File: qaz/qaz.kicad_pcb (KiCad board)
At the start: 2 copper layers, 227.4 x 57.3 mm, 49 parts, among them J1 OLED-128x32, SW1 SW_Push, SW10 SW_Push, SW11 SW_Push, SW12 SW_Push, SW13 SW_Push, SW14 SW_Push, SW15 SW_Push, SW16 SW_Push, SW17 SW_Push, SW18 SW_Push, SW19 SW_Push, SW2 SW_Push, SW20 SW_Push, SW21 SW_Push, SW22 SW_Push, SW23 SW_Push, SW24 SW_Push, SW25 SW_Push, SW26 SW_Push, SW27 SW_Push, SW28 SW_Push, SW3 SW_Push, SW4 SW_Push, SW5 SW_Push, SW6 SW_Push, SW7 SW_Push, SW8 SW_Push, SW9 SW_Push, U1 rp2040-zero

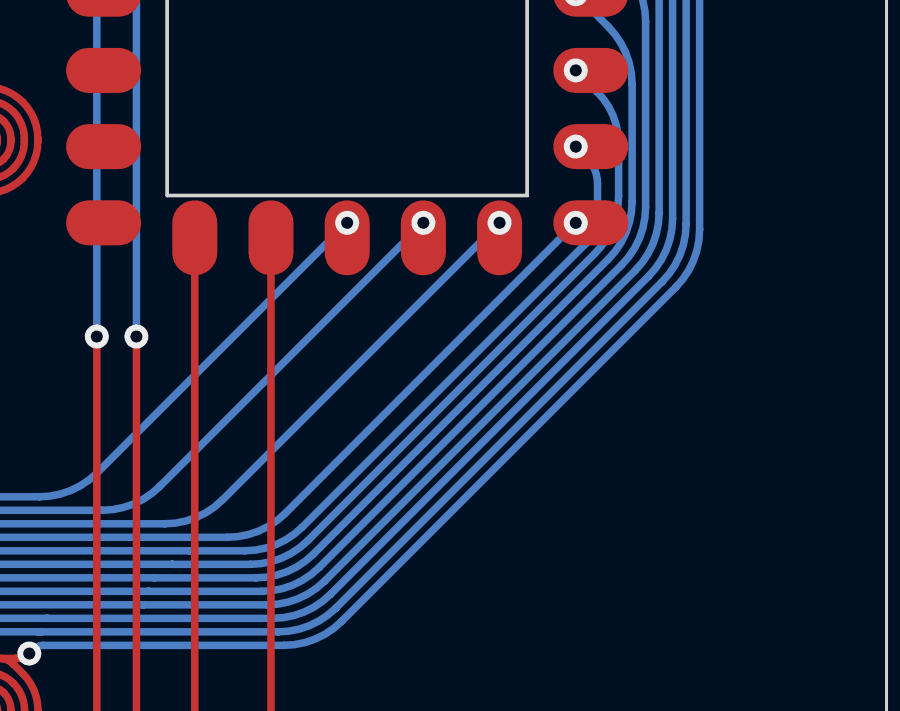
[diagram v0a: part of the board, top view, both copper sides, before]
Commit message: .
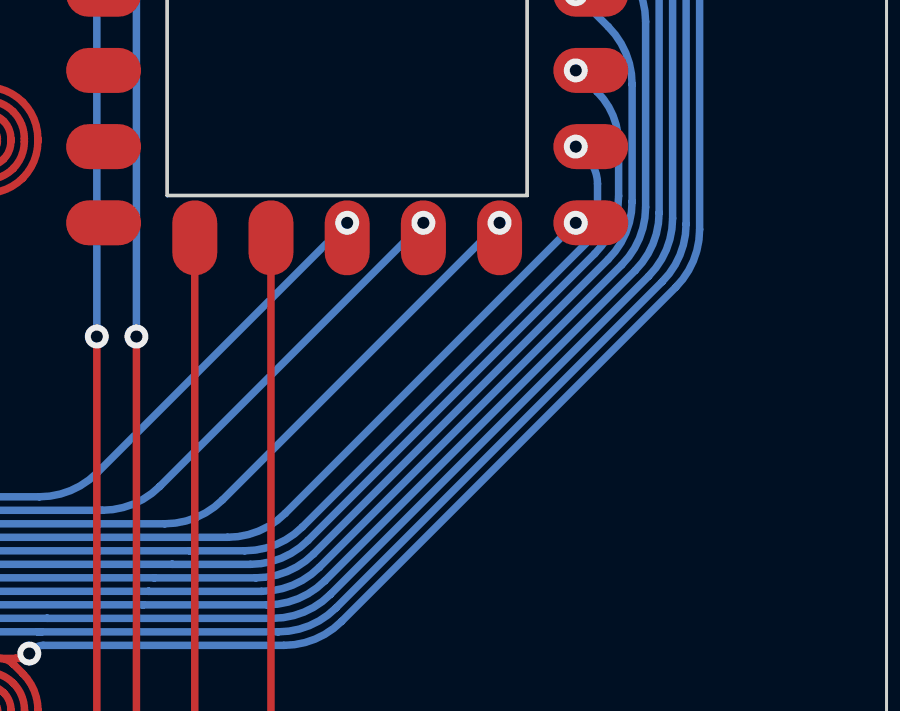
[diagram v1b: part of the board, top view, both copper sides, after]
